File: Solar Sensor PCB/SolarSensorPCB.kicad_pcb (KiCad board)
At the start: 2 copper layers, 28 parts, among them J1 Arduino_Nano_Header, P10 SERIAL, P11 SOFT_SERIAL, P2 BATT, P3 DIO, P4 LOGO1, P5 LOGO2, P6 PCB, P8 AREF, P9 AIO, Q1 PT202C, SW1 UP, SW2 DOWN, SW3 SPST, U1 DS18B20, U2 MCP1702-50, U3 MCP3201

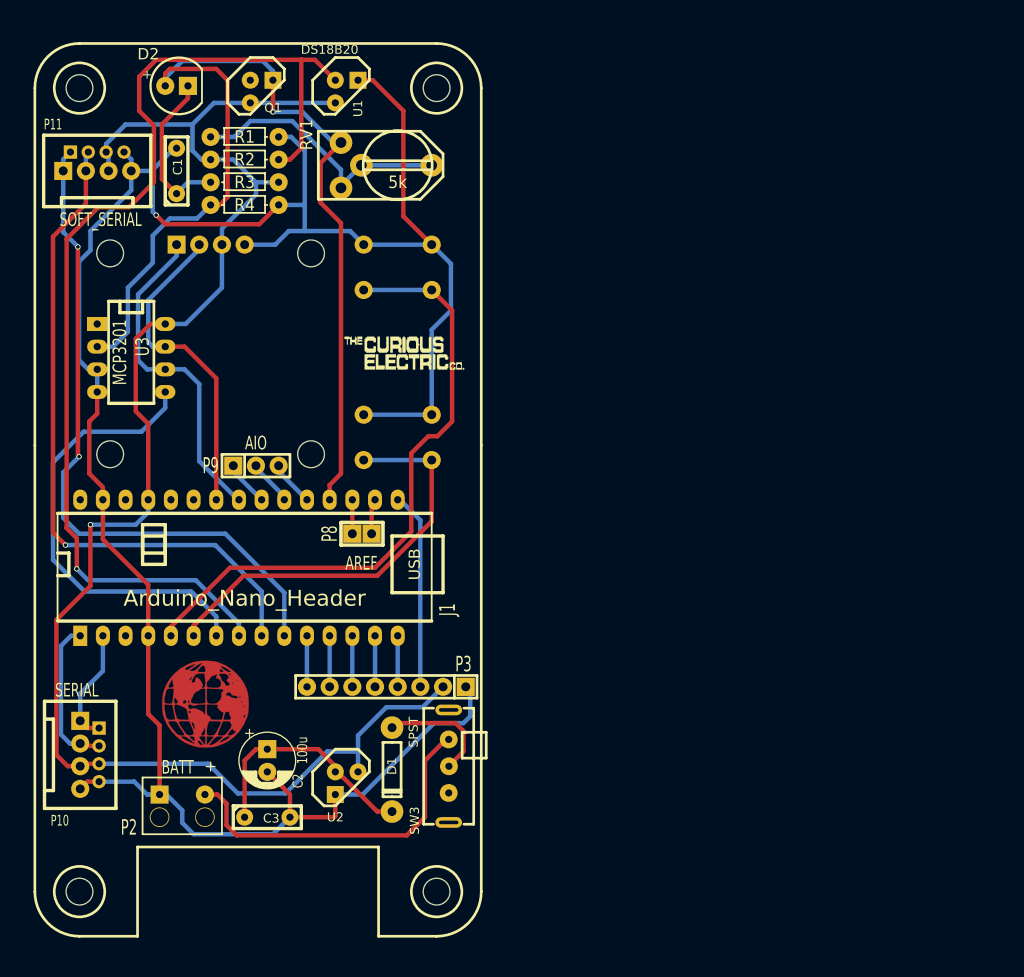
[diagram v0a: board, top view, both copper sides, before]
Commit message: Large update of firmware and PCB
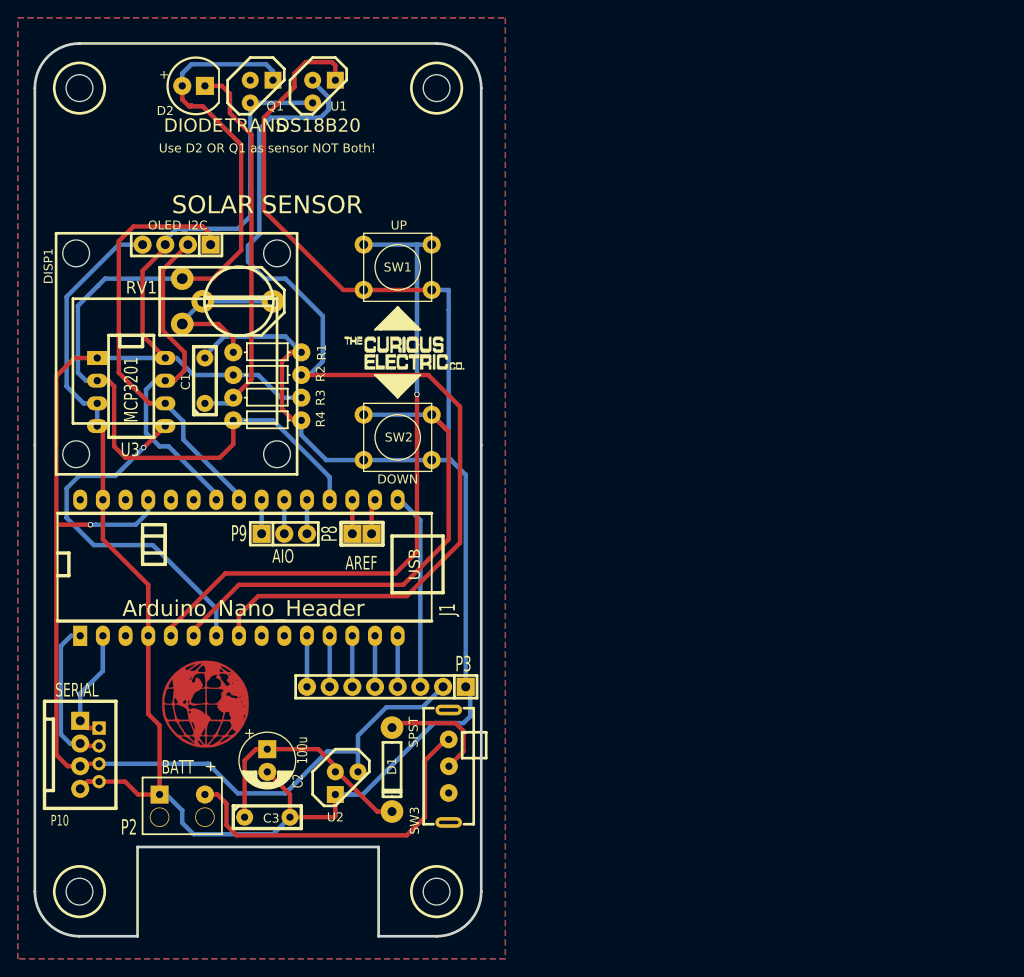
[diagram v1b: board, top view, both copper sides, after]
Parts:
- removed P11: SOFT_SERIAL, matts_components:SIL-4_Grove_SIL
- D2: value PIN -> DIODE
- DISP1, SW1, SW2: moved to F.Cu
- P6: footprint REInnovationFootprint:PCB_50x100mm_PP3_CutOut -> REInnovationFootprint:PCB_50x100mm_PP3_CutOut_EdgeCut
- Q1: value PT202C -> TRANS
- moved R2 24.3 mm to (118.1, 69.2)
- moved R4 24.3 mm to (118.1, 74.3)
- moved R1 24.3 mm to (118.1, 66.7)
- moved R3 24.3 mm to (118.1, 71.8)
- moved C1 23.7 mm to (111.1, 71.1)
- moved RV1 23.4 mm to (113.7, 61.0)
- moved P9 8.26 mm to (120.0, 87.0)
- moved DISP1 3.81 mm to (108.0, 53.3), turned to 0 degrees
- moved U3 3.81 mm to (102.9, 74.9)
- moved U1 2.54 mm to (124.5, 37.5)
- moved D2 1.91 mm to (109.9, 36.8)
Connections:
- J1 pad 10: /Rx_SS -> (no net)
- J1 pad 9: /Tx_SS -> (no net)
- U3 pad 1: (no net) -> +5V
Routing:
- net /Rx_SS: track 75.8 -> 0.00 mm, vias 2 -> 0
- net /Tx_SS: track 75.3 -> 0.00 mm, vias 1 -> 0
- net Net-(C1-Pad1): track 18.3 -> 42.5 mm
- net GND: track 259.2 -> 276.1 mm, vias 1 -> 0
- net Net-(R1-Pad1): track 31.0 -> 19.3 mm
- net /SDA_I2C: track 37.6 -> 49.1 mm
- net /SW_DOWN: track 47.1 -> 58.5 mm
- net /IRR: track 118.7 -> 108.4 mm, vias 1 -> 0
- net /TEMP_DATA: track 121.4 -> 112.0 mm, vias 1 -> 0
- net /CS_ADC: track 50.9 -> 41.8 mm, vias 0 -> 1
- net +5V: track 178.2 -> 185.4 mm
- net /SW_UP: track 70.5 -> 75.7 mm, vias 0 -> 1
- net /SCL_I2C: track 36.2 -> 37.8 mm
- net Net-(J1-Pad20): track 5.13 -> 3.81 mm
- net Net-(J1-Pad22): track 5.13 -> 3.81 mm
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- added copper zone on B.Cu, net GND
- added copper zone on F.Cu, net GND
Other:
- board outline added: 50 x 100 mm
- board text added: "SOLAR SENSOR"
- board text added: "Use D2 OR Q1 as sensor NOT Both!"

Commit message: Updated PCB. Not finished yet!
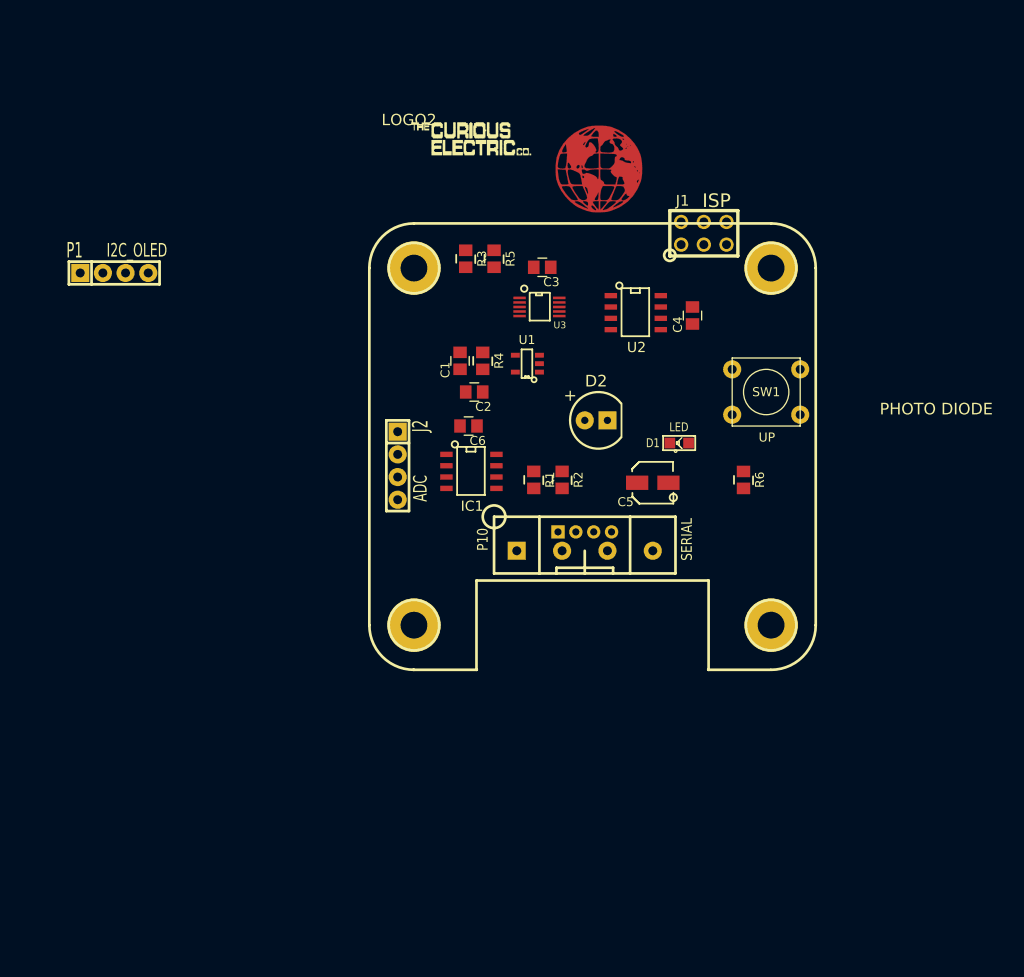
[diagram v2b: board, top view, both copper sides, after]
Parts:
- removed DISP1: OLED_I2C, REInnovationFootprint:TH_OLED1306
- removed P2: BATT, REInnovationFootprint:Batt_Connector_Strain_Relief
- removed P3: DIO, matts_components:SIL-8_lg_pad_1mm
- removed P8: AREF, matts_components:SIL-2_solder_connect
- removed P9: AIO, matts_components:SIL-3_lg_pad_1mm
- removed Q1: TRANS, REInnovationFootprint:TO92-EBC_large_pad
- removed RV1: 5k, REInnovationFootprint:TH_PRESET_Vert_Horiz
- removed SW2: DOWN, REInnovationFootprint:SW_PUSH_SMALL_lg_pad
- removed SW3: SPST, REInnovationFootprint:SW_SPDT_R_Angle_ALIEX
- added C4: 100n, REInnovationFootprint:SM_C_0805, F.Cu at (165.7, 62.6)
- added C5: 100u, REInnovationFootprint:SM_4x5.3, F.Cu at (161.3, 81.3)
- added C6: 100n, REInnovationFootprint:SM_C_0805, F.Cu at (140.7, 74.9)
- added IC1: ATTINY85-P, REInnovationFootprint:SM_SOIC_8, F.Cu at (141.0, 80.6)
- added J2: ADC, REInnovationFootprint:SIL-4_large_pad, F.Cu at (132.7, 79.4)
- added P1: I2C_OLED, REInnovationFootprint:SIL-4_large_pad, F.Cu at (101.0, 57.8)
- added R5: 10k, REInnovationFootprint:SM0805, F.Cu at (143.5, 56.2)
- added R6: 330R, REInnovationFootprint:SM0805, F.Cu at (171.4, 80.9)
- C1: value 100n -> 10n; footprint matts_components:C1_wide_lg_pad -> REInnovationFootprint:SM_C_0805
- C2: value 100u -> 100n; footprint REInnovationFootprint:C_1V7_TH -> REInnovationFootprint:SM_C_0805
- C3: footprint matts_components:C1_wide_lg_pad -> REInnovationFootprint:SM_C_0805
- D1: value 1N5819 -> LED; footprint REInnovationFootprint:TH_Diode_1 -> REInnovationFootprint:SM0805_LED
- D2: value DIODE -> PHOTO DIODE
- J1: value Arduino_Nano_Header -> ISP; footprint REInnovationFootprint:NANO_DIP_30_600 -> REInnovationFootprint:ISP_3x2
- P10: footprint matts_components:SIL-4_Grove_SIL -> REInnovationFootprint:SIL-4_Grove_SCREW
- P6: footprint REInnovationFootprint:PCB_50x100mm_PP3_CutOut_EdgeCut -> REInnovationFootprint:PCB_50x50mm_PP3_Cutout
- R1: value 220 -> 10k; footprint REInnovationFootprint:TH_Resistor_1 -> REInnovationFootprint:SM0805
- R2: value 4K7 -> 10k; footprint REInnovationFootprint:TH_Resistor_1 -> REInnovationFootprint:SM0805
- R3: value 1k -> 10k; footprint REInnovationFootprint:TH_Resistor_1 -> REInnovationFootprint:SM0805
- R4: value 10k -> 47k; footprint REInnovationFootprint:TH_Resistor_1 -> REInnovationFootprint:SM0805
- U1: value DS18B20 -> TSV911xxLx; footprint matts_components:TO92-EBC_large_pad -> REInnovationFootprint:SM_SOT-23-5
- U2: value MCP1702-50 -> LM75B; footprint matts_components:TO92_MC1703 -> REInnovationFootprint:SM_SOIC_8
- U3: value MCP3201 -> ADS1115; footprint REInnovationFootprint:DIP-8_300_ELL -> REInnovationFootprint:SM_MSOP10-0.5
- moved P4 74.4 mm to (155.3, 46.1)
- moved C3 69.4 mm to (148.9, 57.1), turned to 180 degrees
- moved U2 61.3 mm to (159.4, 62.9), turned to 270 degrees
- moved P10 61.0 mm to (153.7, 88.9), turned to 0 degrees
- moved J1 59.6 mm to (167.6, 53.3)
- moved D2 58.6 mm to (154.9, 74.3)
- moved D1 48.4 mm to (164.2, 76.8), turned to 90 degrees
- moved P6 47.9 mm to (129.5, 102.2)
- moved U3 47.6 mm to (148.6, 61.6)
- moved C2 47.3 mm to (141.3, 71.1), turned to 180 degrees
- moved SW1 43.6 mm to (174.0, 71.1)
- moved U1 38.9 mm to (148.6, 67.9), turned to 90 degrees
- moved R2 35.0 mm to (151.1, 80.9)
- moved R1 33.1 mm to (148.0, 80.9)
- moved C1 28.8 mm to (139.7, 67.6)
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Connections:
- C1 pad 1: Net-(C1-Pad1) -> /IRR1+
- C1 pad 2: GND -> Net-(C1-Pad2)
- C2 pad 1: VCC -> GND
- C2 pad 2: GND -> +5V
- C3 pad 1: VCC -> +5V
- D1 pad 1: VCC -> /SW1
- D2 pad 1: Net-(C1-Pad1) -> Net-(C1-Pad2)
- D2 pad 2: /IRR -> GND
- J1 pad 1: /Tx -> /D1
- J1 pad 2: /Rx -> +5V
- J1 pad 3: (no net) -> /D2
- J1 pad 4: GND -> /D0
- J1 pad 5: /SW_UP -> Net-(IC1-Pad1)
- J1 pad 6: /SW_DOWN -> GND
- P4 pad 1: (no net) -> Net-(P4-Pad1)
- R1 pad 1: Net-(R1-Pad1) -> +5V
- R1 pad 2: GND -> /D0
- R2 pad 2: /TEMP_DATA -> /D2
- R3 pad 1: Net-(C1-Pad1) -> +5V
- R3 pad 2: +5V -> Net-(R3-Pad2)
- R4 pad 1: /IRR -> /IRR1+
- R4 pad 2: GND -> Net-(C1-Pad2)
- SW1 pad 1: /SW_UP -> /SW1
- U1 pad 1: +5V -> /IRR1+
- U1 pad 2: /TEMP_DATA -> GND
- U1 pad 3: GND -> Net-(C1-Pad2)
- U3 pad 1: +5V -> Net-(R5-Pad2)
- U3 pad 2: /IRR -> Net-(R3-Pad2)
- U3 pad 4: GND -> /IRR1+
- U3 pad 5: /CS_ADC -> /IRR1-
- U3 pad 6: /SDA_I2C -> Net-(J2-Pad3)
- U3 pad 7: /SCL_I2C -> Net-(J2-Pad2)
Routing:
- net GND: track 276.1 -> 0.00 mm
- net +5V: track 185.4 -> 0.00 mm, vias 1 -> 0
- net /TEMP_DATA: track 112.0 -> 0.00 mm
- net /IRR: track 108.4 -> 0.00 mm
- net /SW_UP: track 75.7 -> 0.00 mm, vias 1 -> 0
- net /SW_DOWN: track 58.5 -> 0.00 mm
- net /SDA_I2C: track 49.1 -> 0.00 mm
- net Net-(C1-Pad1): track 42.5 -> 0.00 mm
- net /CS_ADC: track 41.8 -> 0.00 mm, vias 1 -> 0
- net Net-(P2-Pad2): track 38.8 -> 0.00 mm
- net /SCL_I2C: track 37.8 -> 0.00 mm
- net VCC: track 26.7 -> 0.00 mm
- net Net-(J1-Pad16): track 22.2 -> 0.00 mm
- net Net-(R1-Pad1): track 19.3 -> 0.00 mm
- net /Tx: track 17.3 -> 0.00 mm
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- removed copper zone on B.Cu, net GND
- removed copper zone on F.Cu, net GND
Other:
- board outline removed
- board text removed: "SOLAR SENSOR"
- board text removed: "Use D2 OR Q1 as sensor NOT Both!"
